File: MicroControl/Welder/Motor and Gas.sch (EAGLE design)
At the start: 21 parts, among them IC1 4098D, X1 CON-5.08-03P

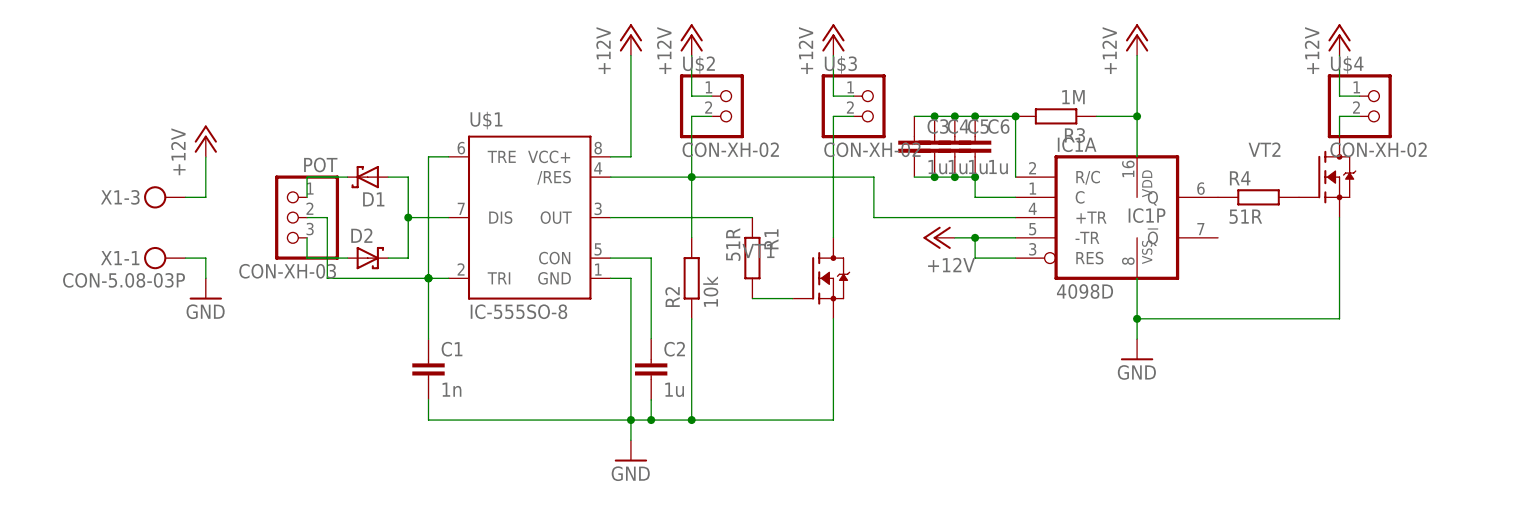
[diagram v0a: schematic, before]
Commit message: Теперь работает
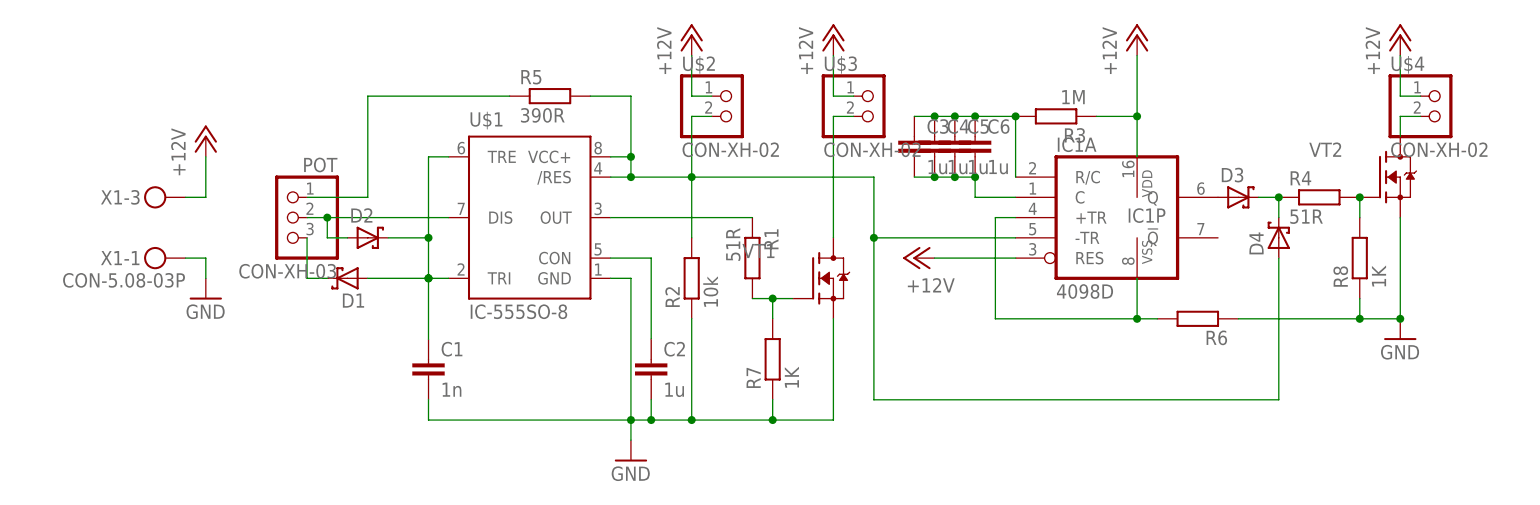
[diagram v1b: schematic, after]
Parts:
- added D3, D4: (no value), Flamberm:DIODE-SH_SOD523
- added R5: 390R, Flamberm:R_1206
- added R6: (no value), Flamberm:R_0805
- added R7, R8: 1K, Flamberm:R_0805
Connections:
- new net N$14: IC1A.+TR, IC1P.VSS, R6.2
- new net N$16: D3.C, D4.C, R4.1
- net +12V: no longer IC1A.-TR, U$1.VCC+
- net GND: now also R6.1, R7.1, R8.1; no longer IC1P.VSS
- net N$12: now also D3.A; no longer R4.1
- net N$13: now also R8.2
- net N$2: now also D1.A, D2.C; no longer POT.2
- net N$4: now also D2.A, POT.2; no longer D1.A, D2.C
- net N$5: now also D1.C; no longer D2.A
- net N$6: now also R5.1; no longer D1.C
- net N$8: now also R7.2
- net N$9: now also D4.A, IC1A.-TR, R5.2, U$1.VCC+; no longer IC1A.+TR
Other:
- moved on the sheet: D1, D2, R4, U$4, VT2
